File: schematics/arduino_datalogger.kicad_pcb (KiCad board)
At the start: 2 copper layers, 95 x 50 mm, 9 parts, among them J1 SD card module, J2 RTC module, J3 Screw_Terminal_01x03, SW1 SW_Push

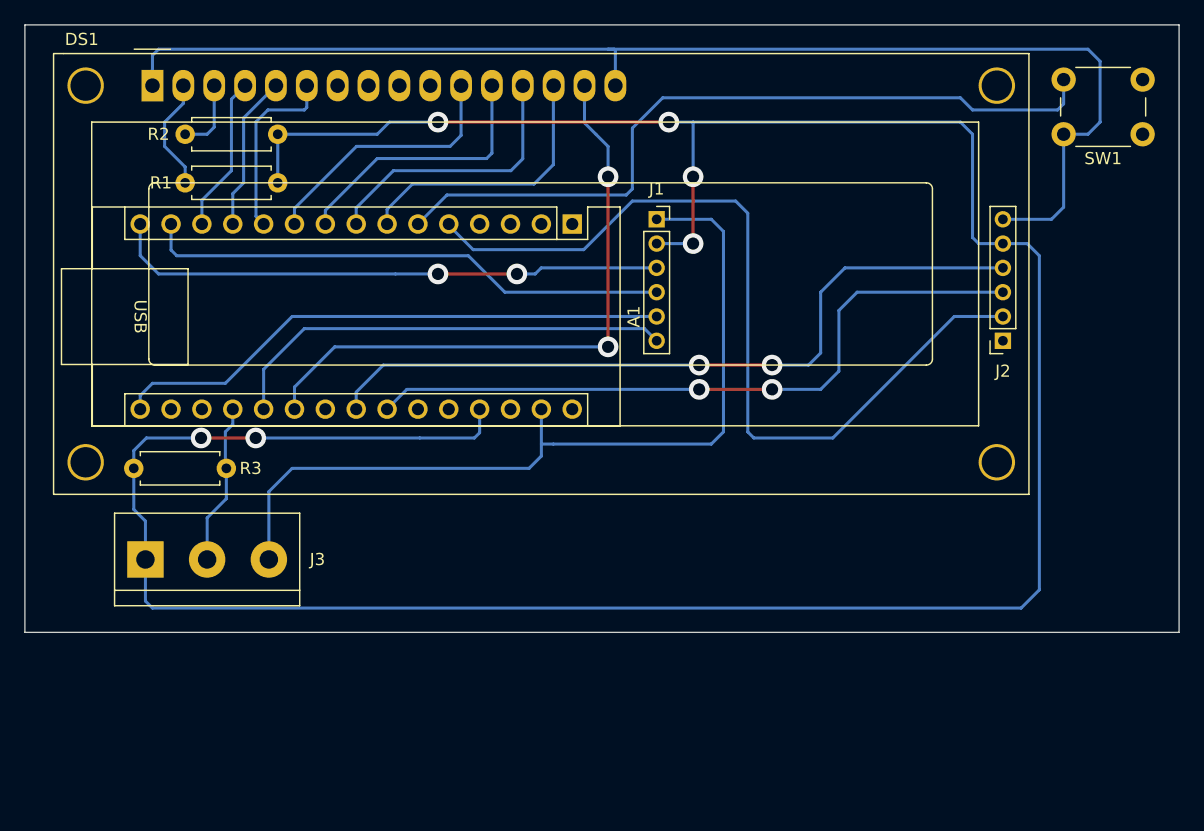
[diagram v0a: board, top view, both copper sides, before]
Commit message: Teniendo en cuenta las medidas reales de los modulos
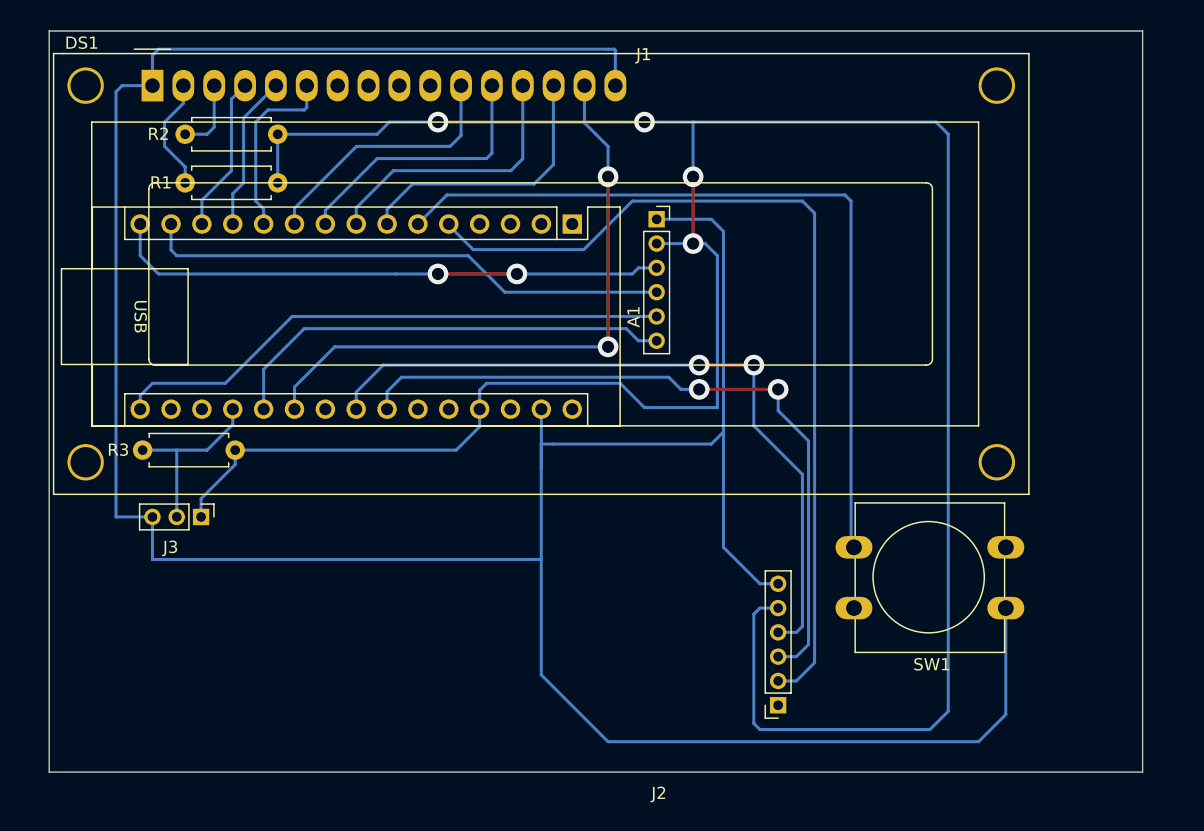
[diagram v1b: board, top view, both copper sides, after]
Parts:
- J3: value Screw_Terminal_01x03 -> DHT; footprint TerminalBlock:TerminalBlock_bornier-3_P5.08mm -> Connector_PinHeader_2.00mm:PinHeader_1x03_P2.00mm_Vertical
- SW1: footprint Button_Switch_THT:SW_PUSH_6mm -> Button_Switch_THT:SW_PUSH-12mm
- moved SW1 40.6 mm to (172.7, 97.0)
- moved J2 35.2 mm to (154.0, 105.0)
- moved R3 8.48 mm to (109.3, 84.0), turned to 180 degrees
- moved J3 5.76 mm to (106.5, 89.5), turned to -90 degrees
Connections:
- A1 pad 4: GND -> unconnected-(A1-GND-Pad4)
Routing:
- net GND: track 175.4 -> 248.6 mm
- net +5V: track 235.5 -> 214.8 mm, vias 6 -> 4
- net SQW: track 71.0 -> 73.7 mm
- net Net-(A1-D3): track 63.0 -> 65.4 mm
- net SCL: track 57.6 -> 59.5 mm
- net /DHTDATA: track 13.3 -> 15.1 mm
- net SDA: track 61.8 -> 60.4 mm
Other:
- board size 95 x 50 mm -> 90 x 61 mm
